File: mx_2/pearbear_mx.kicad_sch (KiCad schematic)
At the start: 20 parts, among them J1 rj11, SW1 SW_Push, SW10 SW_Push, SW11 SW_Push, SW12 SW_Push, SW13 SW_Push, SW14 SW_Push, SW15 SW_Push, SW16 SW_Push, SW17 SW_Push, SW2 SW_Push, SW3 SW_Push, SW4 SW_Push, SW5 SW_Push, SW6 SW_Push, SW7 SW_Push, SW8 SW_Push, SW9 SW_Push, U1 ProMicro-kbd-rev

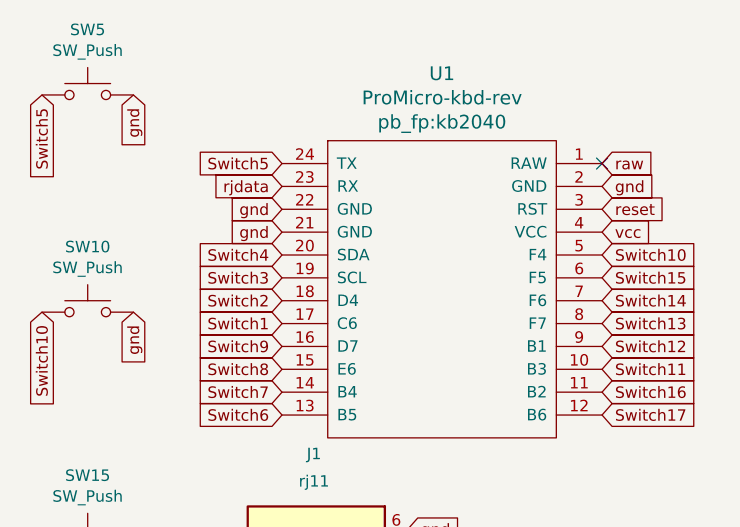
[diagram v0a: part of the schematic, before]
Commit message: hi
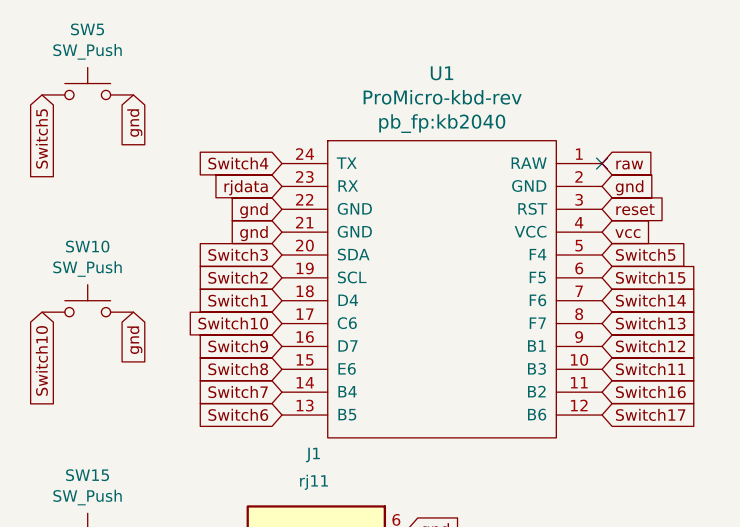
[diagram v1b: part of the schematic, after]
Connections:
- net Switch1: now also U1.18 (D4); no longer U1.17 (C6)
- net Switch10: now also U1.17 (C6); no longer U1.5 (F4)
- net Switch2: now also U1.19 (SCL); no longer U1.18 (D4)
- net Switch3: now also U1.20 (SDA); no longer U1.19 (SCL)
- net Switch4: now also U1.24 (TX); no longer U1.20 (SDA)
- net Switch5: now also U1.5 (F4); no longer U1.24 (TX)
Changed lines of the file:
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@@
 		)
 	)
-	(global_label "Switch4"
+	(global_label "Switch3"
 		(shape input)
 		(at 194.31 74.93 180)
@@
 		)
 	)
-	(global_label "Switch2"
+	(global_label "Switch1"
 		(shape input)
 		(at 194.31 80.01 180)
@@
 		)
 	)
-	(global_label "Switch10"
+	(global_label "Switch5"
 		(shape input)
 		(at 229.87 74.93 0)
@@
 		)
 	)
+	(global_label "Switch10"
+		(shape input)
+		(at 194.31 82.55 180)
+		(effects
+			(font
+				(size 1.27 1.27)
+			)
+			(justify right)
+		)
+		(property "Intersheetrefs" "${INTERSHEET_REFS}"
+			(at 194.31 82.55 0)
+			(effects
+				(font
+					(size 1.27 1.27)
+				)
+				(hide yes)
+			)
+		)
+	)
+	(global_label "raw"
+		(shape input)
+		(at 229.87 64.77 0)
+		(effects
+			(font
+				(size 1.27 1.27)
+			)
+			(justify left)
+		)
+		(property "Intersheetrefs" "${INTERSHEET_REFS}"
+			(at 229.87 64.77 0)
+			(effects
+				(font
+					(size 1.27 1.27)
+				)
+				(hide yes)
+			)
+		)
+	)
+	(global_label "rjdata"
+		(shape input)
+		(at 208.28 113.03 0)
+		(effects
+			(font
+				(size 1.27 1.27)
+			)
+			(justify left)
+		)
+		(property "Intersheetrefs" "${INTERSHEET_REFS}"
+			(at 208.28 113.03 0)
+			(effects
+				(font
+					(size 1.27 1.27)
+				)
+				(hide yes)
+			)
+		)
+	)
+	(global_label "gnd"
+		(shape input)
+		(at 194.31 72.39 180)
+		(effects
+			(font
+				(size 1.27 1.27)
+			)
+			(justify right)
+		)
+		(property "Intersheetrefs" "${INTERSHEET_REFS}"
+			(at 194.31 72.39 0)
+			(effects
+				(font
+					(size 1.27 1.27)
+				)
+				(hide yes)
+			)
+		)
+	)
+	(global_label "Switch8"
+		(shape input)
+		(at 194.31 87.63 180)
+		(effects
+			(font
+				(size 1.27 1.27)
+			)
+			(justify right)
+		)
+		(property "Intersheetrefs" "${INTERSHEET_REFS}"
+			(at 194.31 87.63 0)
+			(effects
+				(font
+					(size 1.27 1.27)
+				)
+				(hide yes)
+			)
+		)
+	)
+	(global_label "Switch13"
+		(shape input)
+		(at 229.87 82.55 0)
+		(effects
+			(font
+				(size 1.27 1.27)
+			)
+			(justify left)
+		)
+		(property "Intersheetrefs" "${INTERSHEET_REFS}"
+			(at 229.87 82.55 0)
+			(effects
+				(font
+					(size 1.27 1.27)
+				)
+				(hide yes)
+			)
+		)
+	)
+	(global_label "Switch9"
+		(shape input)
+		(at 194.31 85.09 180)
+		(effects
+			(font
+				(size 1.27 1.27)
+			)
+			(justify right)
+		)
+		(property "Intersheetrefs" "${INTERSHEET_REFS}"
+			(at 194.31 85.09 0)
+			(effects
+				(font
+					(size 1.27 1.27)
+				)
+				(hide yes)
+			)
+		)
+	)
 	(global_label "Switch1"
 		(shape input)
-		(at 194.31 82.55 180)
-		(effects
-			(font
-				(size 1.27 1.27)
-			)
-			(justify right)
-		)
-		(property "Intersheetrefs" "${INTERSHEET_REFS}"
-			(at 194.31 82.55 0)
-			(effects
-				(font
-					(size 1.27 1.27)
-				)
-				(hide yes)
-			)
-		)
-	)
-	(global_label "raw"
-		(shape input)
-		(at 229.87 64.77 0)
-		(effects
-			(font
-				(size 1.27 1.27)
-			)
-			(justify left)
-		)
-		(property "Intersheetrefs" "${INTERSHEET_REFS}"
-			(at 229.87 64.77 0)
-			(effects
-				(font
-					(size 1.27 1.27)
-				)
-				(hide yes)
-			)
-		)
-	)
-	(global_label "rjdata"
-		(shape input)
-		(at 208.28 113.03 0)
-		(effects
-			(font
-				(size 1.27 1.27)
-			)
-			(justify left)
-		)
-		(property "Intersheetrefs" "${INTERSHEET_REFS}"
-			(at 208.28 113.03 0)
-			(effects
-				(font
-					(size 1.27 1.27)
-				)
-				(hide yes)
-			)
-		)
-	)
-	(global_label "gnd"
-		(shape input)
-		(at 194.31 72.39 180)
-		(effects
-			(font
-				(size 1.27 1.27)
-			)
-			(justify right)
-		)
-		(property "Intersheetrefs" "${INTERSHEET_REFS}"
-			(at 194.31 72.39 0)
-			(effects
-				(font
-					(size 1.27 1.27)
-				)
-				(hide yes)
-			)
-		)
-	)
-	(global_label "Switch8"
-		(shape input)
-		(at 194.31 87.63 180)
-		(effects
-			(font
-				(size 1.27 1.27)
-			)
-			(justify right)
-		)
-		(property "Intersheetrefs" "${INTERSHEET_REFS}"
-			(at 194.31 87.63 0)
-			(effects
-				(font
-					(size 1.27 1.27)
-				)
-				(hide yes)
-			)
-		)
-	)
-	(global_label "Switch13"
-		(shape input)
-		(at 229.87 82.55 0)
-		(effects
-			(font
-				(size 1.27 1.27)
-			)
-			(justify left)
-		)
-		(property "Intersheetrefs" "${INTERSHEET_REFS}"
-			(at 229.87 82.55 0)
-			(effects
-				(font
-					(size 1.27 1.27)
-				)
-				(hide yes)
-			)
-		)
-	)
-	(global_label "Switch9"
-		(shape input)
-		(at 194.31 85.09 180)
-		(effects
-			(font
-				(size 1.27 1.27)
-			)
-			(justify right)
-		)
-		(property "Intersheetrefs" "${INTERSHEET_REFS}"
-			(at 194.31 85.09 0)
-			(effects
-				(font
-					(size 1.27 1.27)
-				)
-				(hide yes)
-			)
-		)
-	)
-	(global_label "Switch1"
-		(shape input)
 		(at 66.04 76.2 270)
 		(effects
@@
 		)
 	)
-	(global_label "Switch5"
+	(global_label "Switch4"
 		(shape input)
 		(at 194.31 64.77 180)
@@
 		)
 	)
-	(global_label "Switch3"
+	(global_label "Switch2"
 		(shape input)
 		(at 194.31 77.47 180)
